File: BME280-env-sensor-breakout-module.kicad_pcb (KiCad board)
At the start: 2 copper layers, 12 x 10 mm, 6 parts, among them J1 I2C_HEADER, U1 BME280

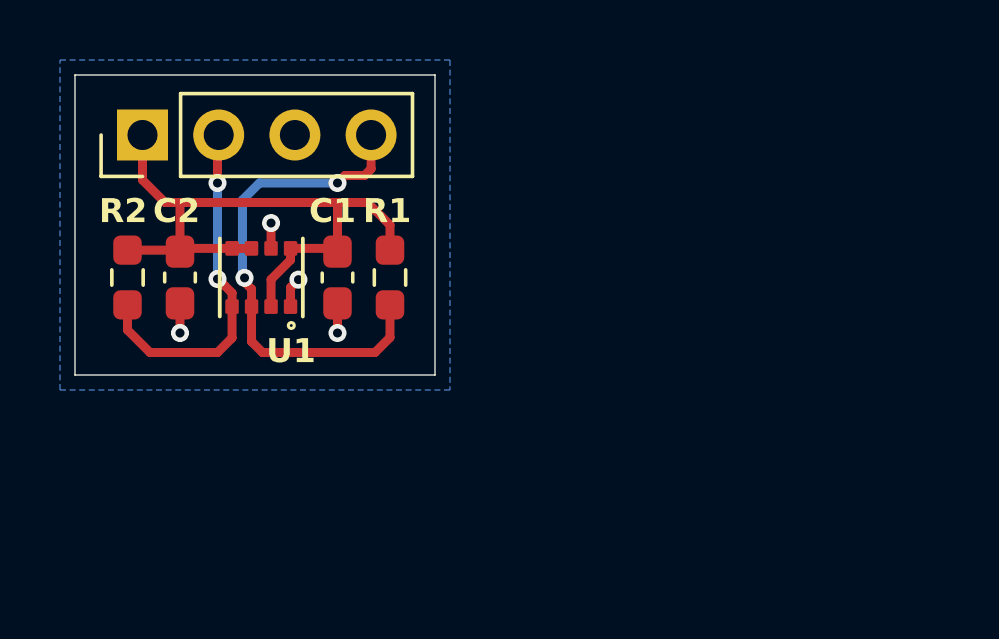
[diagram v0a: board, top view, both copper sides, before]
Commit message: added images
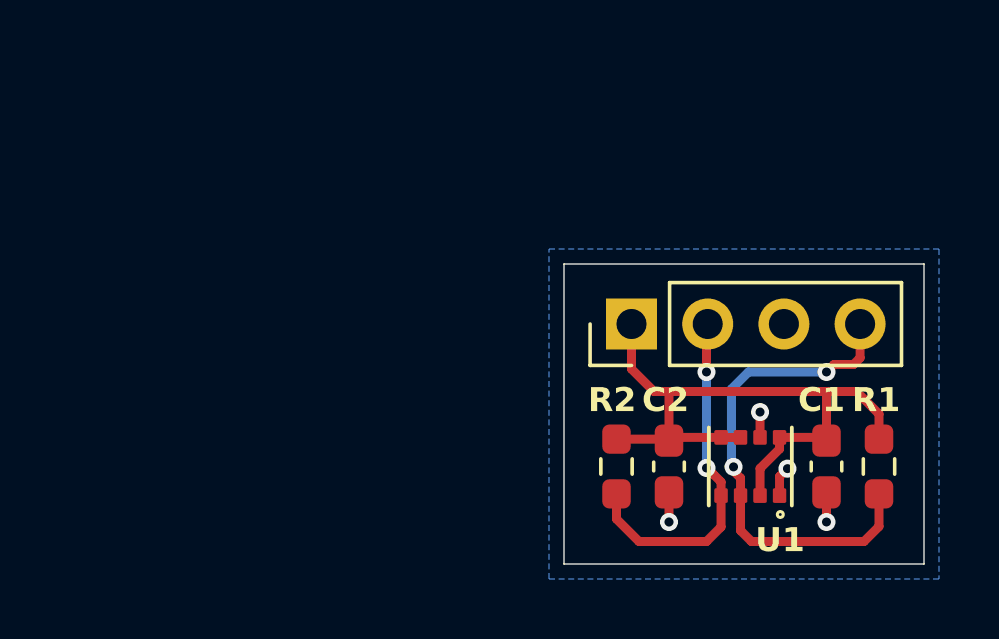
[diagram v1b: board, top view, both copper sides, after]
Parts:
- moved C1 17.5 mm to (155.1, 103.0)
- moved C2 17.5 mm to (149.8, 103.0)
- moved J1 17.5 mm to (148.6, 98.3)
- moved R1 17.5 mm to (156.8, 103.0)
- moved R2 17.5 mm to (148.1, 103.0)
- moved U1 17.5 mm to (152.5, 103.0)
